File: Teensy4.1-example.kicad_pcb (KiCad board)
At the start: 4 copper layers, 61.5 x 47.5 mm, 80 parts, among them IC1 MIMXRT1062DVJ6B, J1 Conn_01x11_Male, J2 Conn_01x11_Male, J3 Conn_01x12_Male, J4 Conn_01x11_Male, J5 Conn_01x11_Male, J6 Conn_01x03_Male, J7 Conn_01x03_Male, P2 D26, Q1 Q_PMOS_GDS, U1 opto_APA102-2020, U2 MAX1562, U3 W25Q64JVXGIM, U4 MKL02Z32VFG4, Y1 Crystal_GND23, Y2 Crystal

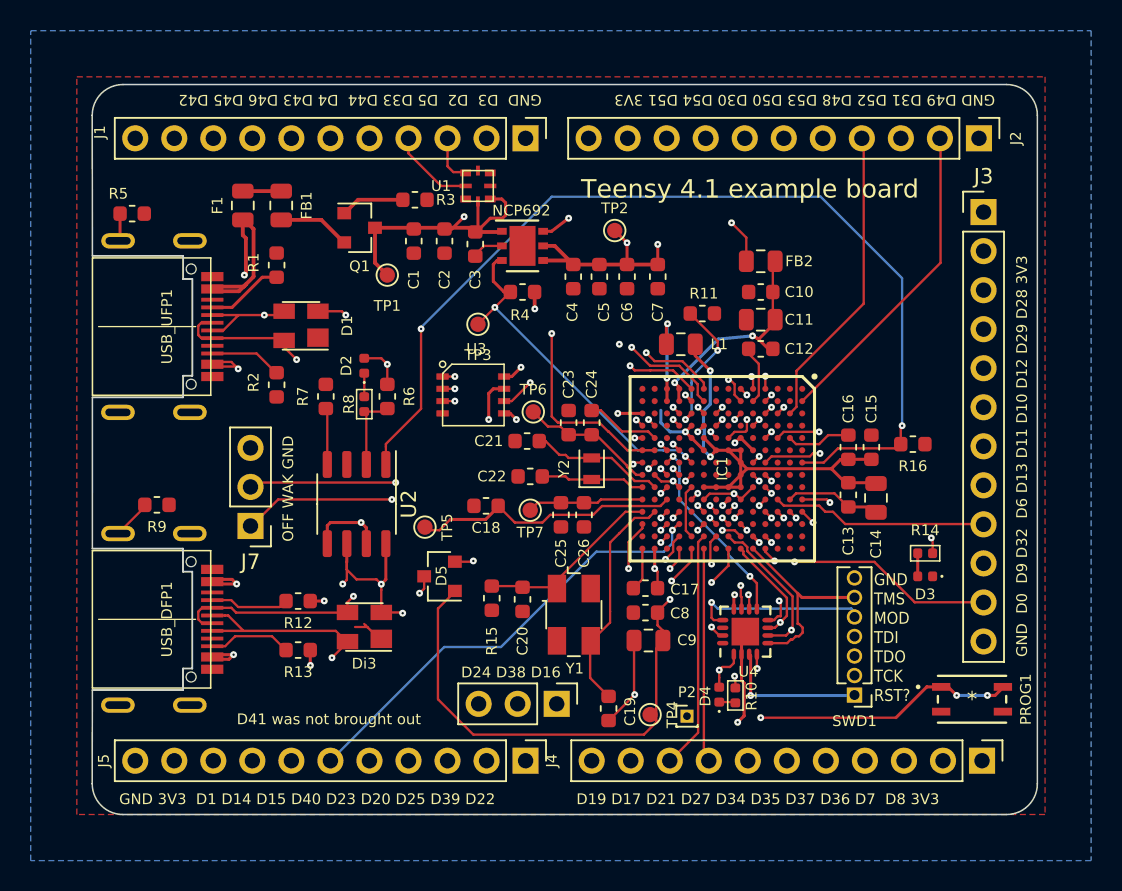
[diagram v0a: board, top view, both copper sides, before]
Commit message: Modified
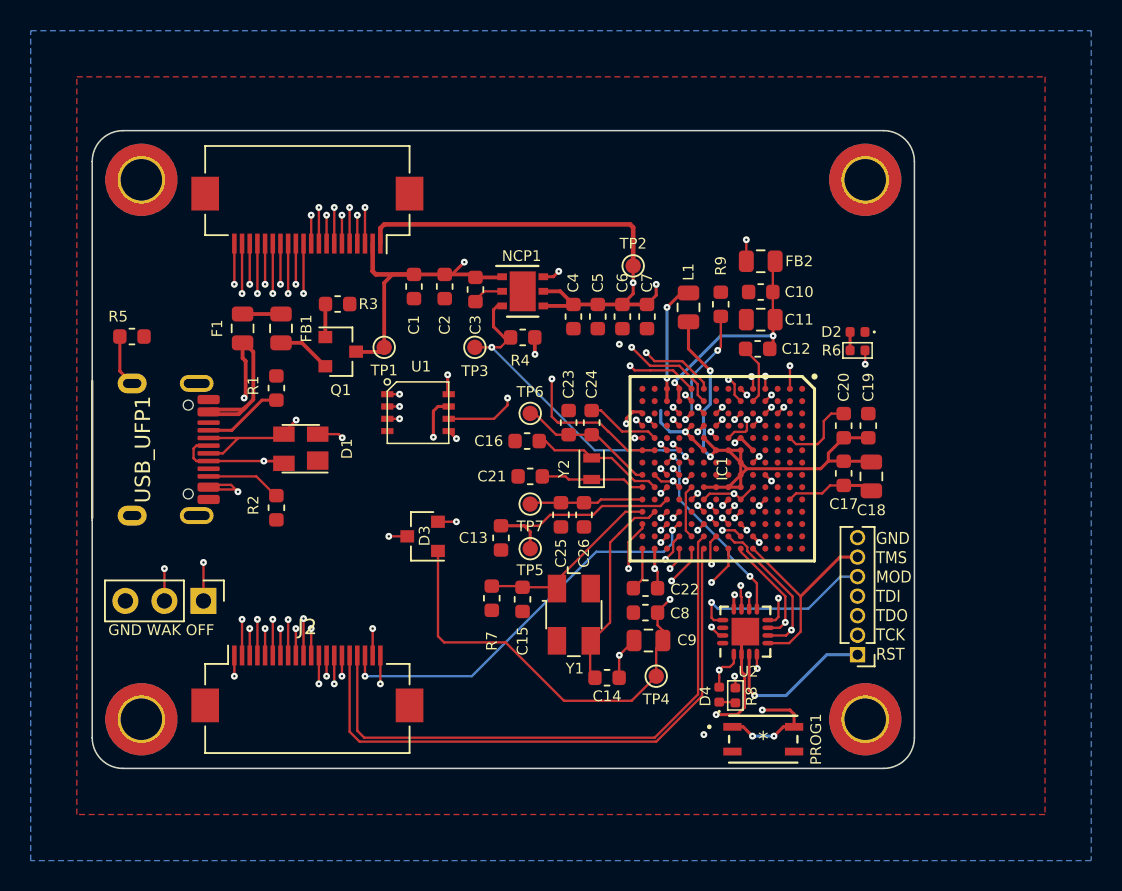
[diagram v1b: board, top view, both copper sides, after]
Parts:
- removed the D2 at (70.7, 92.8)
- removed Di3: SP0503BAHT, Package_TO_SOT_SMD:SOT-143
- removed the J3 at (111.0, 82.8)
- removed J4, J5: Conn_01x11_Male, Connector_PinHeader_2.54mm:PinHeader_1x11_P2.54mm_Vertical
- removed J6: Conn_01x03_Male, Connector_PinHeader_2.54mm:PinHeader_1x03_P2.54mm_Vertical
- removed P2: D26, Connector_PinHeader_1.00mm:PinHeader_1x01_P1.00mm_Vertical
- removed R12, R13: 56k, Resistor_SMD:R_0603_1608Metric
- removed R16: 100k, Resistor_SMD:R_0603_1608Metric
- removed the R6 at (72.2, 94.8)
- removed the R7 at (68.2, 94.8)
- removed the R8 at (70.7, 95.3)
- removed the R9 at (57.2, 101.8)
- removed the U1 at (78.1, 81.1)
- removed the U2 at (70.2, 101.8)
- removed USB_DFP1: USB_C_Receptacle_USB2.0, USB-C-Power-tester:TYPE-C-31-M-14
- added H1: MountingHole, MountingHole:MountingHole_2.7mm_M2.5_DIN965_Pad_TopBottom, F.Cu at (103.3, 80.7)
- added H2: MountingHole, MountingHole:MountingHole_2.7mm_M2.5_DIN965_Pad_TopBottom, F.Cu at (103.3, 115.8)
- added H3: MountingHole, MountingHole:MountingHole_2.7mm_M2.5_DIN965_Pad_TopBottom, F.Cu at (56.2, 115.8)
- added H4: MountingHole, MountingHole:MountingHole_2.7mm_M2.5_DIN965_Pad_TopBottom, F.Cu at (56.2, 80.7)
- J1, J2: value Conn_01x11_Male -> Conn_01x20; footprint Connector_PinHeader_2.54mm:PinHeader_1x11_P2.54mm_Vertical -> Connector_FFC-FPC:Hirose_FH12-20S-0.5SH_1x20-1MP_P0.50mm_Horizontal
- Q1: value Q_PMOS_GDS -> Q_PMOS_GDS_DMP3125L
- USB_UFP1: footprint USB-C-Power-tester:TYPE-C-31-M-14 -> acheron_Connectors:USB_C_Receptacle_Hroparts_TYPE-C-31-M-12
- moved J2 56.3 mm to (67.0, 113.5), turned to 0 degrees
- moved D2 16.5 mm to (102.8, 90.6)
- moved J1 15.1 mm to (67.0, 83.0), turned to 180 degrees
- moved R6 13.9 mm to (102.8, 91.8)
- moved PROG1 13.8 mm to (96.7, 117.1)
- moved USB_UFP1 9.76 mm to (61.3, 98.2)
- moved R3 8.44 mm to (69.0, 88.8)
- moved Q1 8.16 mm to (69.2, 91.9)
- moved D1 8.00 mm to (66.6, 98.2)
- moved F1 8.00 mm to (62.8, 90.4)
- moved FB1 8.00 mm to (65.3, 90.4)
- moved R1 8.00 mm to (65.0, 94.2)
- moved R2 8.00 mm to (65.0, 102.0)
- moved R5 8.00 mm to (55.6, 90.9)
- moved TP5 6.99 mm to (81.5, 104.7)
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- renumbered C18 to C13, C19 to C14, C20 to C15, C21 to C16, C13 to C17, C14 to C18, C15 to C19, C16 to C20, C22 to C21, C17 to C22, D3 to D2, D5 to D3, J7 to J3, NCP692 to NCP1, R14 to R6, R15 to R7, R10 to R8, R11 to R9, U3 to U1, U4 to U2
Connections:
- IC1 pad A10: /D9 -> unconnected-(IC1-GPIO_B0_11-PadA10)
- IC1 pad A11: /D8 -> unconnected-(IC1-GPIO_B1_00-PadA11)
- IC1 pad A2: /D49 -> unconnected-(IC1-GPIO_EMC_27-PadA2)
- IC1 pad A7: Net-(IC1-PadA7) -> unconnected-(IC1-GPIO_EMC_40-PadA7)
- IC1 pad B1: unconnected-(IC1-PadB1) -> /R1
- IC1 pad B11: /D7 -> unconnected-(IC1-GPIO_B1_01-PadB11)
- IC1 pad B3: /D52 -> unconnected-(IC1-GPIO_EMC_26-PadB3)
- IC1 pad C10: /D32 -> unconnected-(IC1-GPIO_B0_12-PadC10)
- IC1 pad C11: /D36 -> unconnected-(IC1-GPIO_B1_02-PadC11)
- IC1 pad C3: /D31 -> /R2
- IC1 pad C5: /D29 -> unconnected-(IC1-GPIO_EMC_31-PadC5)
- IC1 pad D1: /D50 -> /R5
- IC1 pad D11: /D37 -> unconnected-(IC1-GPIO_B1_03-PadD11)
- IC1 pad D13: /D35 -> unconnected-(IC1-GPIO_B1_12-PadD13)
- IC1 pad D14: /D34 -> unconnected-(IC1-GPIO_B1_13-PadD14)
- IC1 pad D2: /D53 -> /R4
- IC1 pad D3: /D48 -> /R3
- IC1 pad D5: /D28 -> unconnected-(IC1-GPIO_EMC_32-PadD5)
- IC1 pad D7: /D10 -> unconnected-(IC1-GPIO_B0_00-PadD7)
- IC1 pad D9: /D6 -> unconnected-(IC1-GPIO_B0_10-PadD9)
- IC1 pad E1: /D54 -> /R7
- IC1 pad E4: /D30 -> /R6
- IC1 pad E7: /D12 -> unconnected-(IC1-GPIO_B0_01-PadE7)
- IC1 pad E8: /D11 -> unconnected-(IC1-GPIO_B0_02-PadE8)
- IC1 pad F1: /D51 -> /R8
- IC1 pad F2: /D2 -> /R10
- IC1 pad G11: /D0 -> /L0
- IC1 pad G12: /D26_A12 -> /L11
- IC1 pad G5: /D3 -> /R9
- IC1 pad H11: /D39_A15 -> /L8
- IC1 pad H12: /D38_A14 -> /L9
- IC1 pad H13: /D22_A8 -> /L10
- IC1 pad H3: /D5 -> /R11
- IC1 pad H4: /D33 -> /R12
- IC1 pad H5: /D4 -> /R14
- IC1 pad J1: /D43 -> /R15
- IC1 pad J11: /D19_A5 -> /L13
- IC1 pad J12: /D17_A3 -> /L12
- IC1 pad J13: /D21_A7 -> /L16
- IC1 pad J14: /D27_A13 -> /L15
- IC1 pad J2: /D46 -> /R16
- IC1 pad J3: /D44 -> /R13
- IC1 pad J4: /D45 -> /R17
- IC1 pad K1: /D42 -> /R18
- IC1 pad K10: /D16_A2 -> /L14
- IC1 pad K11: /D18_A4 -> unconnected-(IC1-GPIO_AD_B1_01-PadK11)
- IC1 pad K12: /D41_A17 -> unconnected-(IC1-GPIO_AD_B1_05-PadK12)
- IC1 pad K14: /D24_A10 -> /L7
- IC1 pad L11: /D14_A0 -> /L2
- IC1 pad L12: /D40_A16 -> /L17
- IC1 pad L13: /D20_A6 -> /L5
- IC1 pad L14: /D25_A11 -> /L6
- IC1 pad M11: /D1 -> /L1
- IC1 pad M12: /D15_A1 -> /L3
- IC1 pad M13: /D23_A9 -> /L4
- IC1 pad N7: /USB2_DN -> unconnected-(IC1-USB_OTG2_DN-PadN7)
- IC1 pad P7: /USB2_DP -> unconnected-(IC1-USB_OTG2_DP-PadP7)
- J1 pad 1: GND -> +3V3
- J1 pad 10: /D45 -> /R8
- J1 pad 11: /D42 -> /R9
- J1 pad 2: /D3 -> +5V
- J1 pad 3: /D2 -> /R1
- J1 pad 4: /D5 -> /R2
- J1 pad 5: /D33 -> /R3
- J1 pad 6: /D44 -> /R4
- J1 pad 7: /D4 -> /R5
- J1 pad 8: /D43 -> /R6
- J1 pad 9: /D46 -> /R7
- J2 pad 1: GND -> /L0
- J2 pad 10: /D51 -> /L9
- J2 pad 11: +3V3 -> /L10
- J2 pad 2: /D49 -> /L1
- J2 pad 3: /D31 -> /L2
- J2 pad 4: /D52 -> /L3
- J2 pad 5: /D48 -> /L4
- J2 pad 6: /D53 -> /L5
- J2 pad 7: /D50 -> /L6
- J2 pad 8: /D30 -> /L7
- J2 pad 9: /D54 -> /L8
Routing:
- net Net-(IC1-PadA7): track 64.6 -> 0.00 mm, vias 2 -> 0
- net /L0: track 0.00 -> 62.0 mm, vias 0 -> 3
- net /D45: track 44.9 -> 0.00 mm, vias 2 -> 0
- net /D42: track 43.3 -> 0.00 mm, vias 1 -> 0
- net /L11: track 0.00 -> 42.5 mm, vias 0 -> 2
- net /L13: track 0.00 -> 40.7 mm, vias 0 -> 2
- net /L14: track 0.00 -> 40.5 mm, vias 0 -> 2
- net /L12: track 0.00 -> 40.0 mm, vias 0 -> 2
- net /D46: track 39.8 -> 0.00 mm, vias 1 -> 0
- net /R3: track 0.00 -> 39.3 mm, vias 0 -> 2
- net /R17: track 0.00 -> 39.1 mm, vias 0 -> 3
- net /R6: track 0.00 -> 39.0 mm, vias 0 -> 2
- net /L15: track 0.00 -> 39.0 mm
- net /R9: track 0.00 -> 39.0 mm, vias 0 -> 2
- net /L16: track 0.00 -> 38.9 mm
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- removed copper zone on In1.Cu, net +5VL
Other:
- board size 61.5 x 47.5 mm -> 53.5 x 41.5 mm
- board text added: "GND TMS MOD TDI TDO TCK RST"
- board text added: "GND WAK OFF"
- board text removed: "D19 D17 D21 D27 D34 D35 D37 D36 D7 D8 3V3"
- board text removed: "D24 D38 D16"
- board text removed: "D41 was not brought out"
- board text removed: "GND 3V3 D1 D14 D15 D40 D23 D20 D25 D39 D22"
- board text removed: "GND D0 D9 D32 D6 D13 D11 D10 D12 D29 D28 3V3"
- board text removed: "GND D3 D2 D5 D33 D44 D4 D43 D46 D45 D42"
- board text removed: "GND D49 D31 D52 D48 D53 D50 D30 D54 D51 3V3"
- board text removed: "GND TMS MOD TDI TDO TCK RST?"
- board text removed: "OFF WAK GND"
- board text removed: "Teensy 4.1 example board"
- board text removed: "Teensy 4.1 example board Feel free to use this as a starting point for your own boards, but pls do the fanout smarter (D41 got trapped and is not broken out). The board includes the required parts - MIMXRT1062DVJ6B (Arm Cortex M7 @ 600 Mhz) - MKL02Z32VFG4 (must be purchased from PJRC) - W25Q64JVXGIM (8Mb spi Flash) Optional parts (not in PJRC's design) - USB Type C for power & debug - USB Type C 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"
